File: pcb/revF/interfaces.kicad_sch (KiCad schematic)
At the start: 49 parts, among them CON3 VGA, CON7 SOUND, J4 UART2, J7 ESP-BUS, J8 TAPE IN, J9 TAPE OUT, Q2 BC847, U10 ESP-12E, U11 TDA1543, U16 LM311, U21 AMS1117-3.3, U7 TXB0104PW

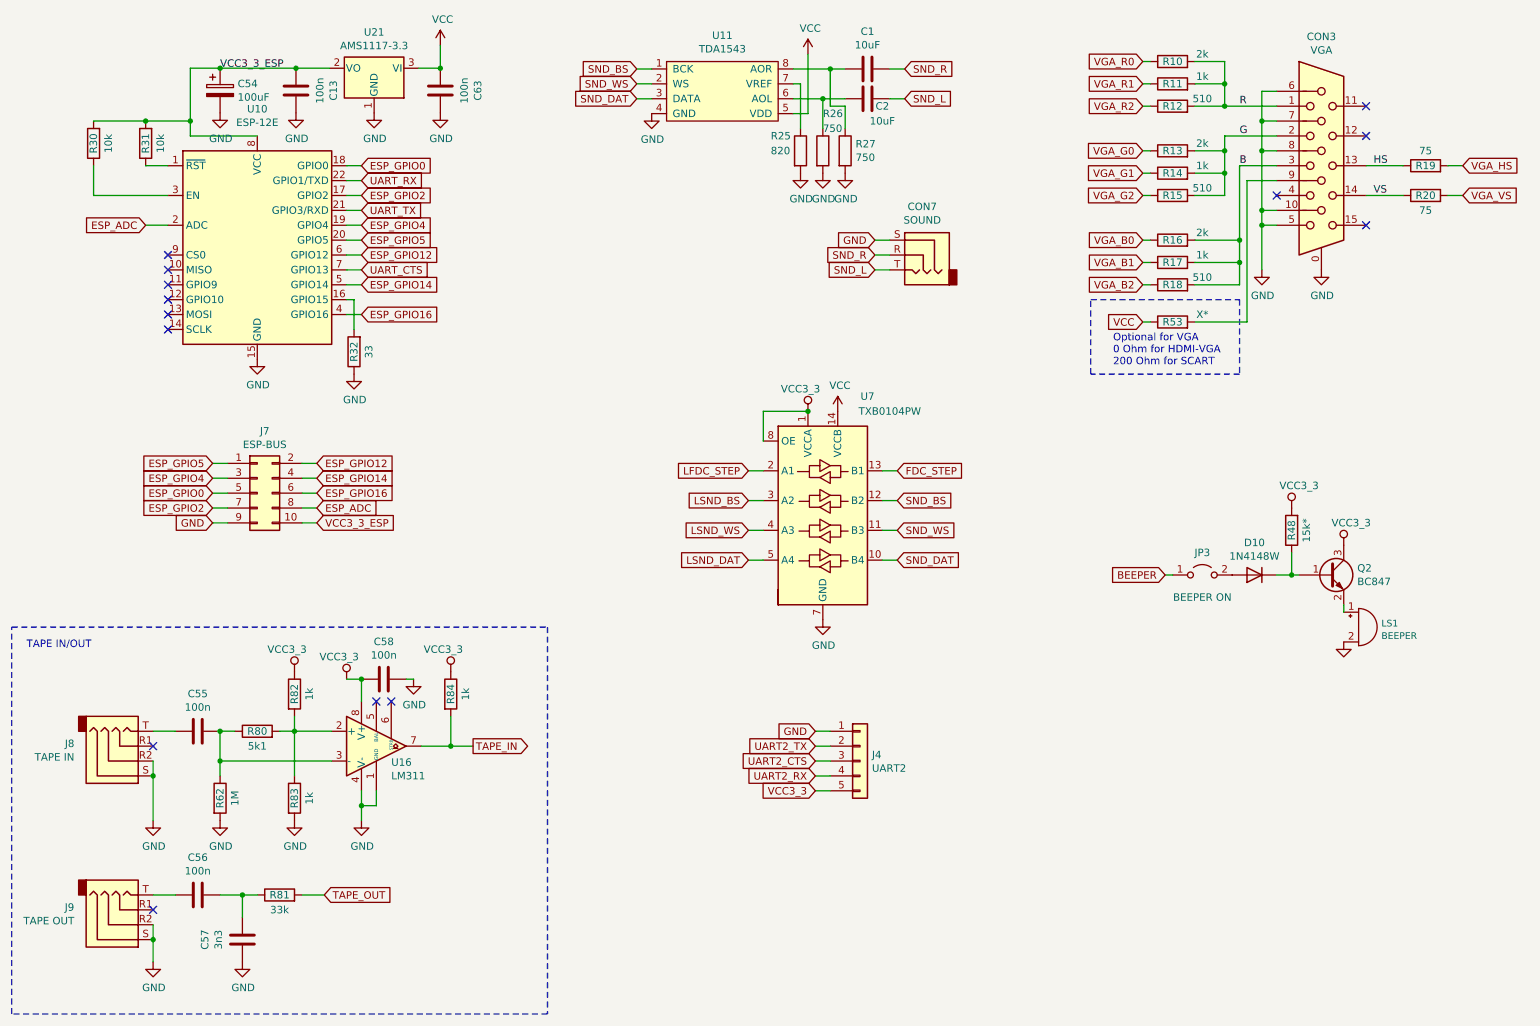
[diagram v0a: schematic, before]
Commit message: New schematics / revF
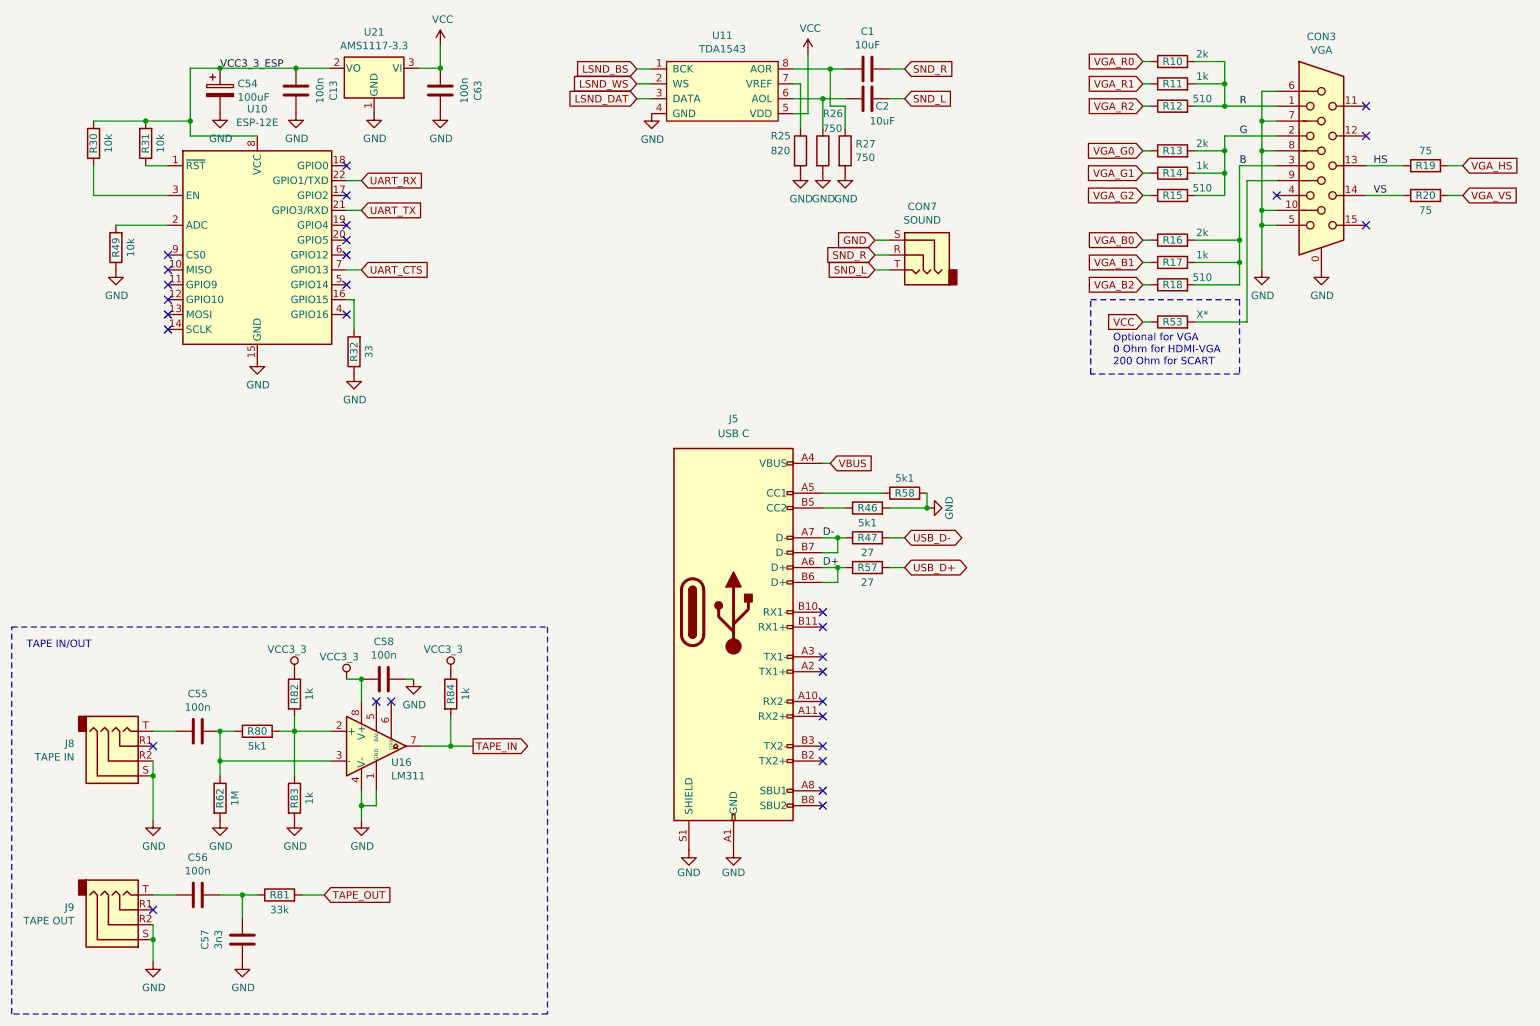
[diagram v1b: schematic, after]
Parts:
- removed D10: 1N4148W, Diode_SMD:D_SOD-123, symbol Diode:1N4148W
- removed J4: UART2, Connector_PinHeader_2.54mm:PinHeader_1x05_P2.54mm_Vertical, symbol Connector_Generic:Conn_01x05
- removed J7: ESP-BUS, Connector_PinHeader_2.54mm:PinHeader_2x05_P2.54mm_Vertical, symbol Connector_Generic:Conn_02x05_Odd_Even
- removed JP3: BEEPER ON, Connector_PinHeader_2.54mm:PinHeader_1x02_P2.54mm_Vertical, symbol Jumper:Jumper_2_Open
- removed LS1: BEEPER, Buzzer_Beeper:Buzzer_12x9.5RM7.6, symbol Device:Buzzer
- removed Q2: BC847, Package_TO_SOT_SMD:SOT-23, symbol Transistor_BJT:BC847
- removed R48: 15k*, Resistor_SMD:R_0805_2012Metric_Pad1.20x1.40mm_HandSolder, symbol Device:R
- removed U7: TXB0104PW, Package_SO:TSSOP-14_4.4x5mm_P0.65mm, symbol Logic_LevelTranslator:TXB0104PW
- added J5: USB C, Connector_USB:USB_C_Receptacle_XKB_U262-16XN-4BVC11, symbol Connector:USB_C_Receptacle
- added R46, R58: 5k1, Resistor_SMD:R_0805_2012Metric_Pad1.20x1.40mm_HandSolder, symbol Device:R
- added R47, R57: 27, Resistor_SMD:R_0805_2012Metric_Pad1.20x1.40mm_HandSolder, symbol Device:R
- added R49: 10k, Resistor_SMD:R_0805_2012Metric_Pad1.15x1.40mm_HandSolder, symbol Device:R
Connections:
- net SND_BS is gone; now on net LSND_BS: U11.1 (BCK)
- net SND_DAT is gone; now on net LSND_DAT: U11.3 (DATA)
- net SND_WS is gone; now on net LSND_WS: U11.2 (WS)
- net GND: now also J5.A1 (GND), J5.A12 (GND), J5.B1 (GND), J5.B12 (GND), J5.S1 (SHIELD), R46.2, R49.1, R58.2
- net ESP_ADC: no longer names the net of U10.2 (ADC)
- net ESP_ADC: now also R49.2
- net ESP_GPIO0: no longer names the net of U10.18 (GPIO0)
- net ESP_GPIO12: no longer names the net of U10.6 (GPIO12)
- net ESP_GPIO14: no longer names the net of U10.5 (GPIO14)
- net ESP_GPIO16: no longer names the net of U10.4 (GPIO16)
- net ESP_GPIO2: no longer names the net of U10.17 (GPIO2)
- net ESP_GPIO4: no longer names the net of U10.19 (GPIO4)
- net ESP_GPIO5: no longer names the net of U10.20 (GPIO5)
- new net: J5.B5 (CC2), R46.1
- new net: J5.A5 (CC1), R58.1
- new net D+: J5.A6 (D+), J5.B6 (D+), R57.1
- new net D-: J5.A7 (D-), J5.B7 (D-), R47.1
- new net USB_D+: R57.2
- new net USB_D-: R47.2
- new net VBUS: J5.A4 (VBUS), J5.A9 (VBUS), J5.B4 (VBUS), J5.B9 (VBUS)
- no-connect marks 14 -> 31
